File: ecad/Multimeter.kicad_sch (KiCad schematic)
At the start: 14 parts, among them J1 Red Banana Plug, J2 Black Banana Plug, SW1 SW_Push_DPDT, U1 SC0915, U3 MCP6001-OT, U4 MCP3561

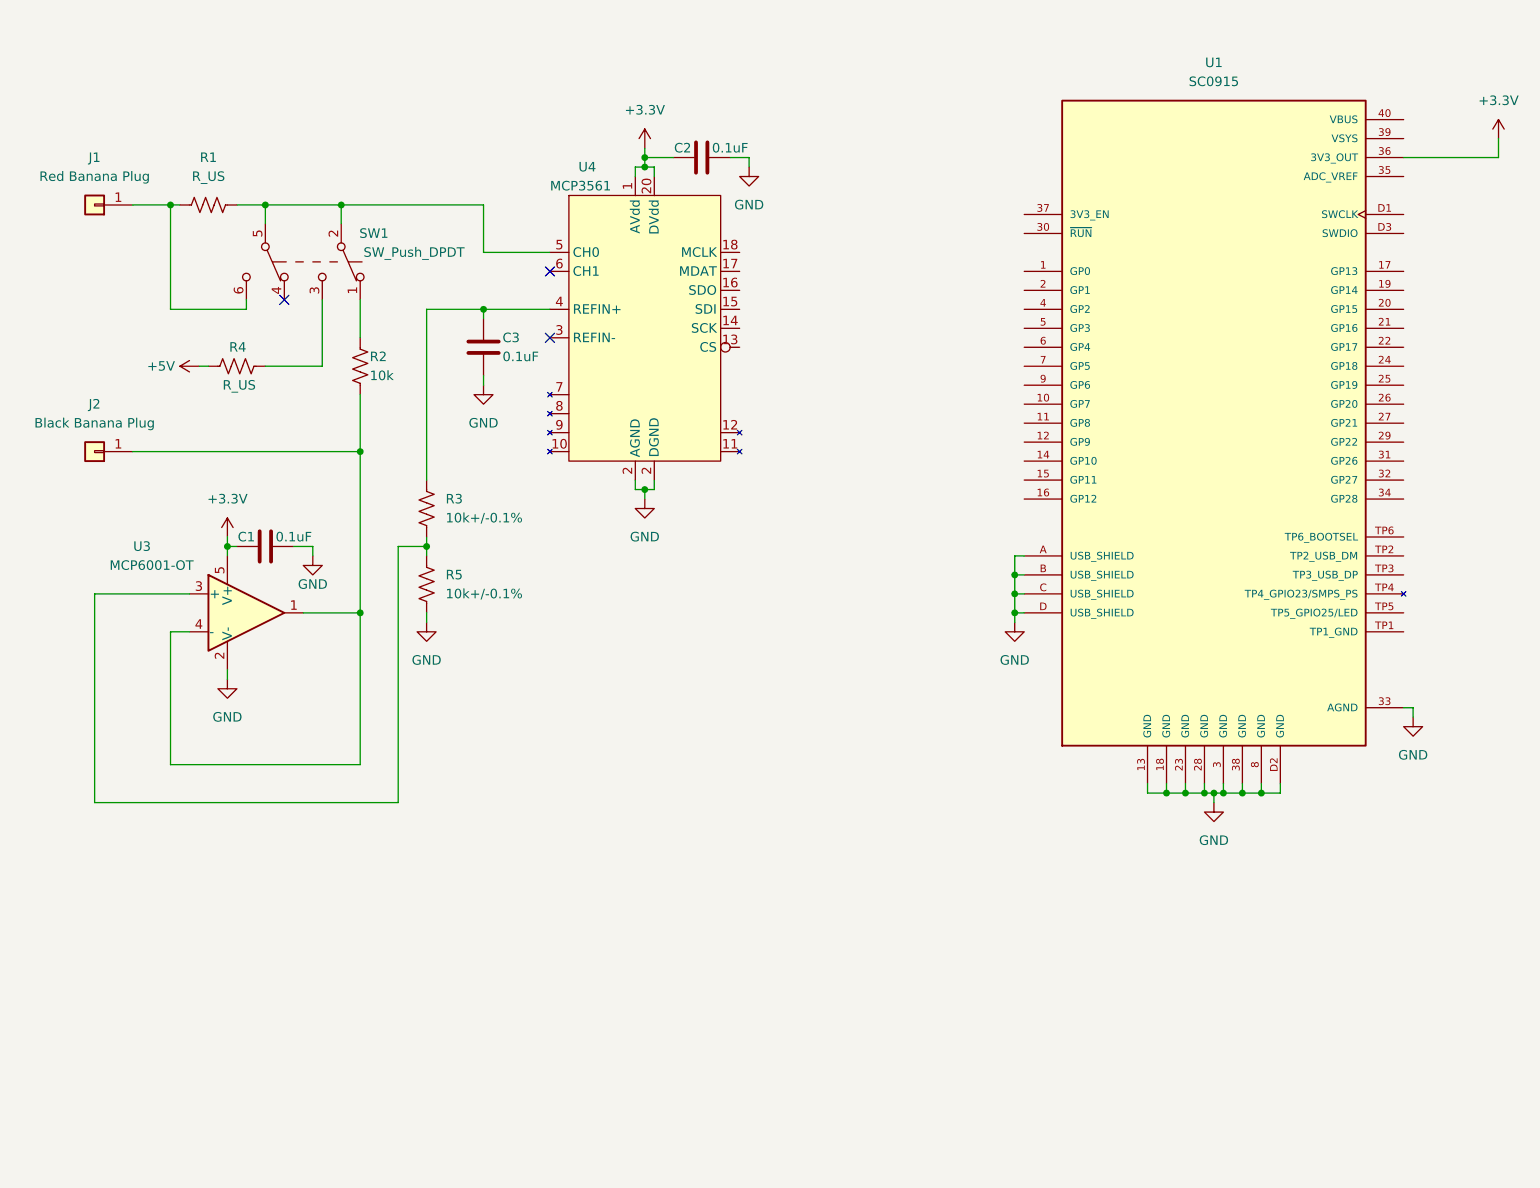
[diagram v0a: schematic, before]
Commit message: stuff
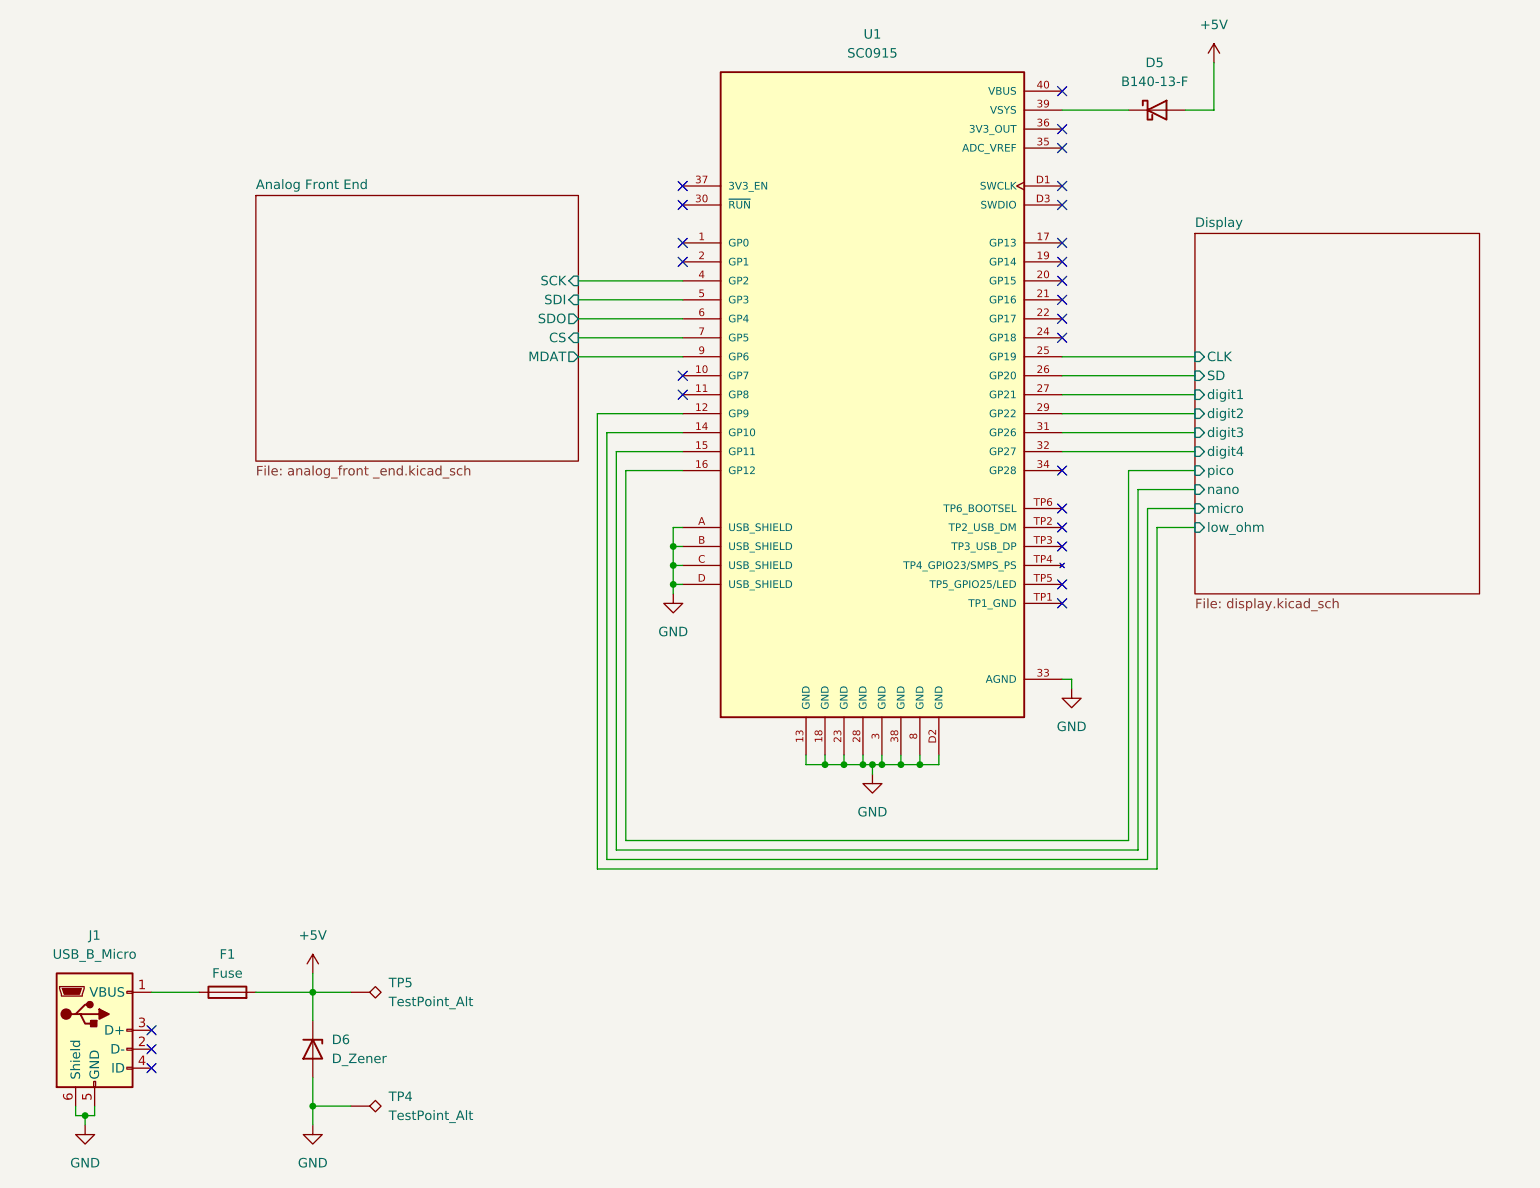
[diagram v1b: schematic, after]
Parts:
- removed C1, C2, C3: 0.1uF, symbol Device:C
- removed J1: Red Banana Plug, symbol Connector_Generic:Conn_01x01
- removed J2: Black Banana Plug, symbol Connector_Generic:Conn_01x01
- removed R1, R4: R_US, symbol Device:R_US
- removed R2: 10k, symbol Device:R_US
- removed R3, R5: 10k+/-0.1%, symbol Device:R_US
- removed SW1: SW_Push_DPDT, symbol Switch:SW_Push_DPDT
- removed U3: MCP6001-OT, Package_TO_SOT_SMD:SOT-23-5, symbol Amplifier_Operational:MCP6001-OT
- removed U4: MCP3561, symbol multimeter_parts:MCP3561
- added D5: B140-13-F, Diode_SMD:D_0805_2012Metric, symbol Device:D_Schottky
- added D6: D_Zener, symbol Device:D_Zener
- added F1: Fuse, Diode_SMD:D_0805_2012Metric, symbol Device:Fuse
- added J1: USB_B_Micro, symbol Connector:USB_B_Micro
- added TP4, TP5: TestPoint_Alt, symbol Connector:TestPoint_Alt
- U1: footprint SC0915:MODULE_SC0915 -> Multimeter:MODULE_SC0915
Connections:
- net +5V: now also D5.2 (A), D6.1 (K), F1.2, TP5.1
- net GND: now also D6.2 (A), J1.5 (GND), J1.6 (Shield), TP4.1
- net Display/low_ohm: now reaches U1.12 (GP9)
- net Display/micro: now reaches U1.14 (GP10)
- net Display/nano: now reaches U1.15 (GP11)
- net Display/pico: now reaches U1.16 (GP12)
- net Display/CLK: now reaches U1.25 (GP19)
- net Display/SD: now reaches U1.26 (GP20)
- net Display/digit1: now reaches U1.27 (GP21)
- net Display/digit2: now reaches U1.29 (GP22)
- net Display/digit3: now reaches U1.31 (GP26)
- net Display/digit4: now reaches U1.32 (GP27)
- net at U1.39 (VSYS): now also D5.1 (K)
- net Analog Front End/SCK: now reaches U1.4 (GP2)
- net Analog Front End/SDI: now reaches U1.5 (GP3)
- net Analog Front End/SDO: now reaches U1.6 (GP4)
- net Analog Front End/CS: now reaches U1.7 (GP5)
- net Analog Front End/MDAT: now reaches U1.9 (GP6)
- net +3.3V: no longer names the net of U1.36 (3V3_OUT)
- new net: F1.1, J1.1 (VBUS)
- no-connect marks 3 -> 26
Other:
- added sheet Analog Front End (analog_front _end.kicad_sch)
- added sheet Display (display.kicad_sch)
- moved on the sheet: U1
